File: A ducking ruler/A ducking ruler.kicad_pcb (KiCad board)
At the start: 2 copper layers, 210 x 40 mm, 32 parts

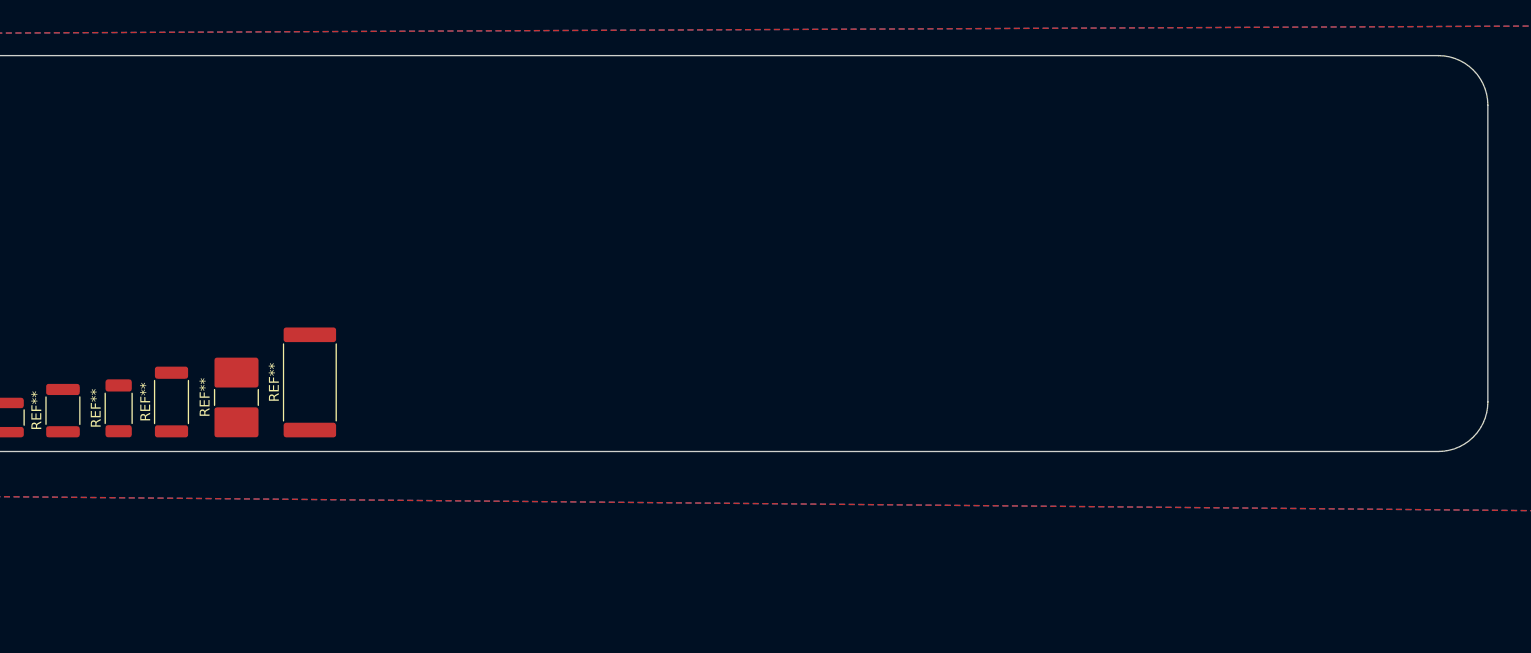
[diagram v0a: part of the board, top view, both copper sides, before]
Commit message: feat: added ducks
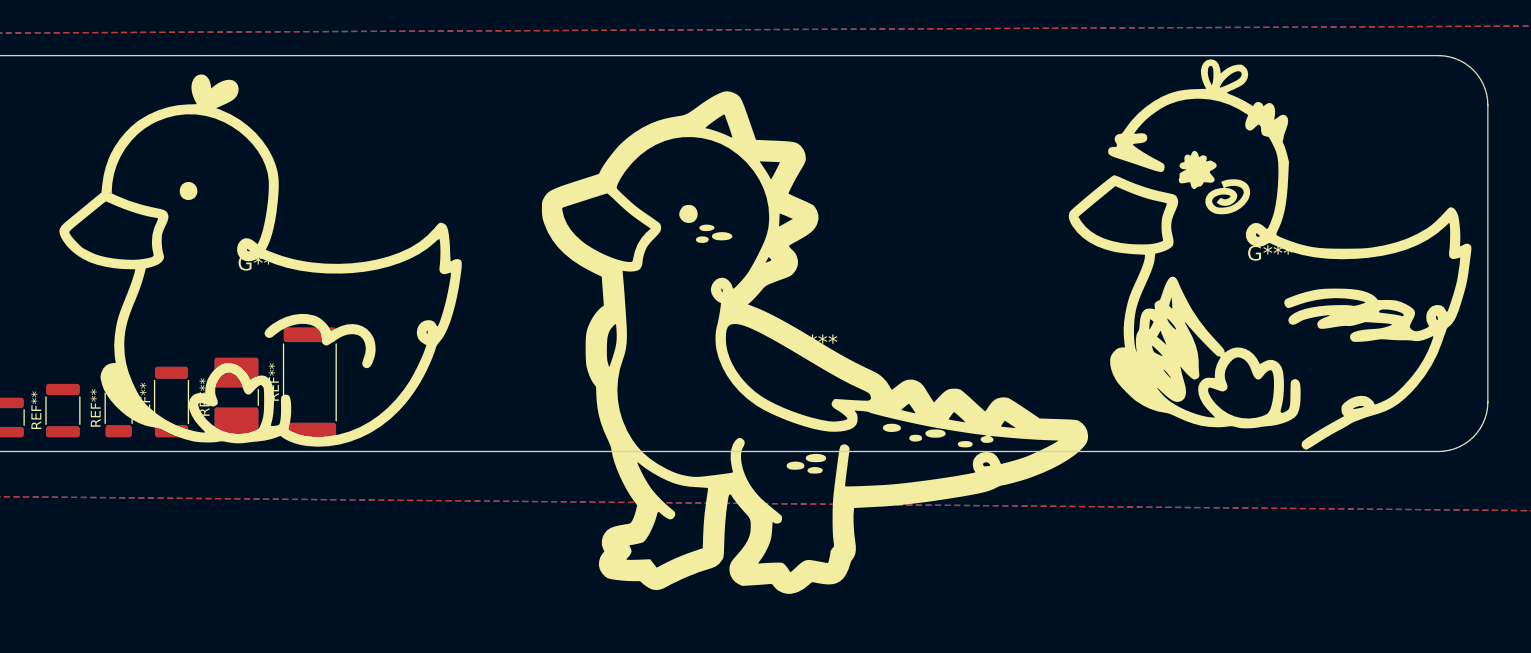
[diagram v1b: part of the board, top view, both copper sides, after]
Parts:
- added G***: LOGO, Angelussss:Doodle_Duck, F.Cu at (233.0, 97.0)
- added G***: LOGO, Angelussss:Basic_Duck, F.Cu at (131.0, 98.0)
- added G***: LOGO, Angelussss:Dino_Duck, F.Cu at (187.0, 106.0)
